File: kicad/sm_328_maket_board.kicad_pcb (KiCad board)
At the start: 2 copper layers, 54.7 x 61.7 mm, 301 parts

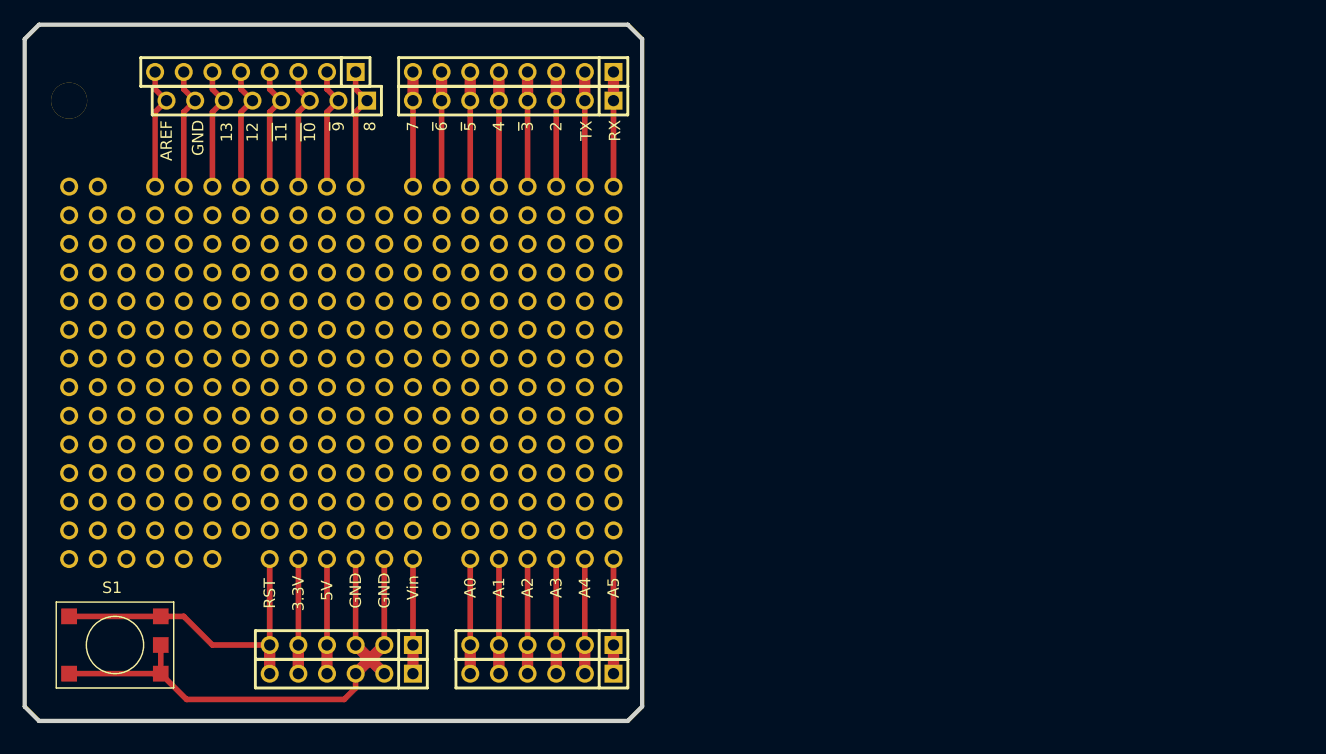
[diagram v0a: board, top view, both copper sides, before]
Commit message: Продолжил разрабатывать макетную плату.
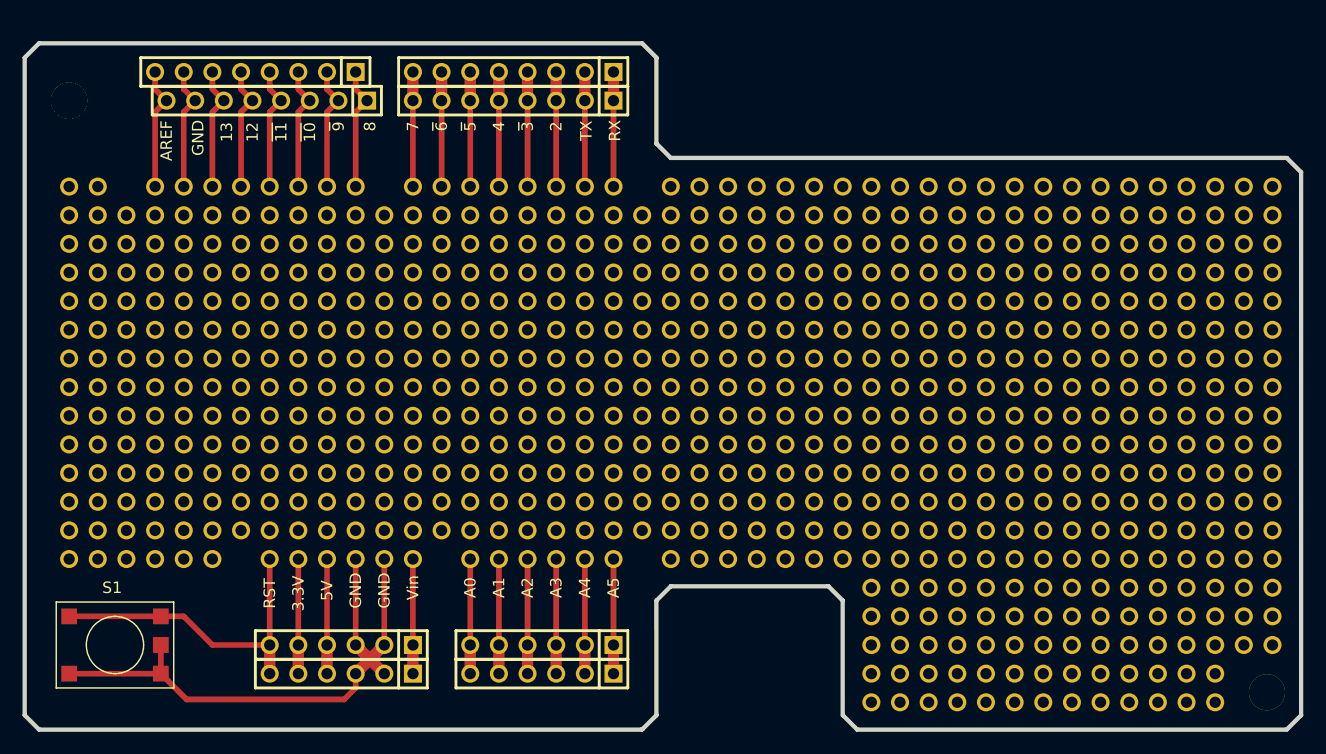
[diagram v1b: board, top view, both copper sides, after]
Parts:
- added G447: P***, 1_pin, F.Cu at (191.0, 139.1)
- added arduino: P***, 1_pin, F.Cu at (175.3, 130.8)
- added arduino: P***, 1_pin, F.Cu at (182.9, 108.0)
- added arduino: P***, 1_pin, F.Cu at (142.2, 123.2)
- added arduino: P***, 1_pin, F.Cu at (193.0, 113.0)
- added arduino: P***, 1_pin, F.Cu at (193.0, 108.0)
- added arduino: P***, 1_pin, F.Cu at (185.4, 97.8)
- added arduino: P***, 1_pin, F.Cu at (154.9, 113.0)
- added arduino: P***, 1_pin, F.Cu at (165.1, 118.1)
- added arduino: P***, 1_pin, F.Cu at (162.6, 113.0)
- added arduino: P***, 1_pin, F.Cu at (180.3, 113.0)
- added arduino: P***, 1_pin, F.Cu at (147.3, 110.5)
- added arduino: P***, 1_pin, F.Cu at (147.3, 108.0)
- added arduino: P***, 1_pin, F.Cu at (167.6, 125.7)
- added arduino: P***, 1_pin, F.Cu at (160.0, 110.5)
- added arduino: P***, 1_pin, F.Cu at (180.3, 118.1)
- added arduino: P***, 1_pin, F.Cu at (149.9, 120.7)
- added arduino: P***, 1_pin, F.Cu at (177.8, 95.2)
- added arduino: P***, 1_pin, F.Cu at (172.7, 120.7)
- added arduino: P***, 1_pin, F.Cu at (188.0, 95.2)
- added arduino: P***, 1_pin, F.Cu at (188.0, 97.8)
- added arduino: P***, 1_pin, F.Cu at (162.6, 100.3)
- added arduino: P***, 1_pin, F.Cu at (144.8, 115.6)
- added arduino: P***, 1_pin, F.Cu at (195.6, 125.7)
- added arduino: P***, 1_pin, F.Cu at (170.2, 130.8)
- added arduino: P***, 1_pin, F.Cu at (147.3, 125.7)
- added arduino: P***, 1_pin, F.Cu at (152.4, 113.0)
- added arduino: P***, 1_pin, F.Cu at (162.6, 135.9)
- added arduino: P***, 1_pin, F.Cu at (170.2, 115.6)
- added arduino: P***, 1_pin, F.Cu at (162.6, 110.5)
- added arduino: P***, 1_pin, F.Cu at (167.6, 113.0)
- added arduino: P***, 1_pin, F.Cu at (165.1, 125.7)
- added arduino: P***, 1_pin, F.Cu at (149.9, 108.0)
- added arduino: P***, 1_pin, F.Cu at (154.9, 108.0)
- added arduino: P***, 1_pin, F.Cu at (170.2, 141.0)
- added arduino: P***, 1_pin, F.Cu at (177.8, 97.8)
- added arduino: P***, 1_pin, F.Cu at (185.4, 130.8)
- added arduino: P***, 1_pin, F.Cu at (157.5, 105.4)
- added arduino: P***, 1_pin, F.Cu at (167.6, 141.0)
- added arduino: P***, 1_pin, F.Cu at (166.6, 109.7)
- added arduino: P***, 1_pin, F.Cu at (172.7, 115.6)
- added arduino: P***, 1_pin, F.Cu at (156.5, 109.7)
- added arduino: P***, 1_pin, F.Cu at (180.3, 133.3)
- added arduino: P***, 1_pin, F.Cu at (195.6, 135.9)
- added arduino: P***, 1_pin, F.Cu at (182.9, 95.2)
- added arduino: P***, 1_pin, F.Cu at (190.5, 108.0)
- added arduino: P***, 1_pin, F.Cu at (182.9, 118.1)
- added arduino: P***, 1_pin, F.Cu at (160.0, 120.7)
- added arduino: P***, 1_pin, F.Cu at (160.0, 133.3)
- added arduino: P***, 1_pin, F.Cu at (182.9, 123.2)
- added arduino: P***, 1_pin, F.Cu at (185.4, 123.2)
- added arduino: P***, 1_pin, F.Cu at (165.1, 105.4)
- added arduino: P***, 1_pin, F.Cu at (160.0, 95.2)
- added arduino: P***, 1_pin, F.Cu at (195.6, 100.3)
- added arduino: P***, 1_pin, F.Cu at (188.0, 110.5)
- added arduino: P***, 1_pin, F.Cu at (154.9, 97.8)
- added arduino: P***, 1_pin, F.Cu at (190.5, 113.0)
- added arduino: P***, 1_pin, F.Cu at (152.4, 100.3)
- added arduino: P***, 1_pin, F.Cu at (152.4, 95.2)
- added arduino: P***, 1_pin, F.Cu at (190.5, 141.0)
- added arduino: P***, 1_pin, F.Cu at (172.7, 123.2)
- added arduino: P***, 1_pin, F.Cu at (177.8, 133.3)
- added arduino: P***, 1_pin, F.Cu at (180.3, 128.3)
- added arduino: P***, 1_pin, F.Cu at (160.0, 138.4)
- added arduino: P***, 1_pin, F.Cu at (190.5, 105.4)
- added arduino: P***, 1_pin, F.Cu at (142.2, 110.5)
- added arduino: P***, 1_pin, F.Cu at (160.0, 108.0)
- added arduino: P***, 1_pin, F.Cu at (190.5, 115.6)
- added arduino: P***, 1_pin, F.Cu at (142.2, 113.0)
- added arduino: P***, 1_pin, F.Cu at (185.4, 120.7)
- added arduino: P***, 1_pin, F.Cu at (152.4, 102.9)
- added arduino: P***, 1_pin, F.Cu at (195.6, 108.0)
- added arduino: P***, 1_pin, F.Cu at (185.4, 95.2)
- added arduino: P***, 1_pin, F.Cu at (195.6, 97.8)
- added arduino: P***, 1_pin, F.Cu at (188.0, 108.0)
- added arduino: P***, 1_pin, F.Cu at (167.6, 135.9)
- added arduino: P***, 1_pin, F.Cu at (139.7, 123.2)
- added arduino: P***, 1_pin, F.Cu at (147.3, 113.0)
- added arduino: P***, 1_pin, F.Cu at (185.4, 118.1)
- added arduino: P***, 1_pin, F.Cu at (165.1, 138.4)
- added arduino: P***, 1_pin, F.Cu at (193.0, 100.3)
- added arduino: P***, 1_pin, F.Cu at (180.3, 105.4)
- added arduino: P***, 1_pin, F.Cu at (185.4, 105.4)
- added arduino: P***, 1_pin, F.Cu at (167.6, 110.5)
- added arduino: P***, 1_pin, F.Cu at (149.9, 128.3)
- added arduino: P***, 1_pin, F.Cu at (193.0, 97.8)
- added arduino: P***, 1_pin, F.Cu at (188.0, 130.8)
- added arduino: P***, 1_pin, F.Cu at (167.6, 133.3)
- added arduino: P***, 1_pin, F.Cu at (167.6, 130.8)
- added arduino: P***, 1_pin, F.Cu at (165.1, 113.0)
- added arduino: P***, 1_pin, F.Cu at (175.3, 138.4)
- added arduino: P***, 1_pin, F.Cu at (175.3, 125.7)
- added arduino: P***, 1_pin, F.Cu at (171.7, 109.7)
- added arduino: P***, 1_pin, F.Cu at (177.8, 141.0)
- added arduino: P***, 1_pin, F.Cu at (147.3, 128.3)
- added arduino: P***, 1_pin, F.Cu at (169.2, 109.7)
- added arduino: P***, 1_pin, F.Cu at (177.8, 105.4)
- added arduino: P***, 1_pin, F.Cu at (160.0, 100.3)
- added arduino: P***, 1_pin, F.Cu at (157.5, 108.0)
- added arduino: P***, 1_pin, F.Cu at (175.3, 123.2)
- added arduino: P***, 1_pin, F.Cu at (185.4, 110.5)
- added arduino: P***, 1_pin, F.Cu at (177.8, 113.0)
- added arduino: P***, 1_pin, F.Cu at (175.3, 95.2)
- added arduino: P***, 1_pin, F.Cu at (142.2, 95.2)
- added arduino: P***, 1_pin, F.Cu at (142.2, 125.7)
- added arduino: P***, 1_pin, F.Cu at (177.8, 115.6)
- added arduino: P***, 1_pin, F.Cu at (188.0, 115.6)
- added arduino: P***, 1_pin, F.Cu at (157.5, 95.2)
- added arduino: P***, 1_pin, F.Cu at (149.9, 113.0)
- added arduino: P***, 1_pin, F.Cu at (185.4, 108.0)
- added arduino: P***, 1_pin, F.Cu at (177.8, 138.4)
- added arduino: P***, 1_pin, F.Cu at (185.4, 125.7)
- added arduino: P***, 1_pin, F.Cu at (157.5, 120.7)
- added arduino: P***, 1_pin, F.Cu at (160.0, 115.6)
- added arduino: P***, 1_pin, F.Cu at (164.1, 109.7)
- added arduino: P***, 1_pin, F.Cu at (184.4, 109.7)
- added arduino: P***, 1_pin, F.Cu at (167.6, 100.3)
- added arduino: P***, 1_pin, F.Cu at (193.0, 125.7)
- added arduino: P***, 1_pin, F.Cu at (165.1, 141.0)
- added arduino: P***, 1_pin, F.Cu at (190.5, 130.8)
- added arduino: P***, 1_pin, F.Cu at (180.3, 108.0)
- added arduino: P***, 1_pin, F.Cu at (175.3, 102.9)
- added arduino: P***, 1_pin, F.Cu at (162.6, 138.4)
- added arduino: P***, 1_pin, F.Cu at (180.3, 120.7)
- added arduino: P***, 1_pin, F.Cu at (152.4, 125.7)
- added arduino: P***, 1_pin, F.Cu at (177.8, 108.0)
- added arduino: P***, 1_pin, F.Cu at (165.1, 123.2)
- added arduino: P***, 1_pin, F.Cu at (182.9, 135.9)
- added arduino: P***, 1_pin, F.Cu at (157.5, 123.2)
- added arduino: P***, 1_pin, F.Cu at (180.3, 141.0)
- added arduino: P***, 1_pin, F.Cu at (182.9, 105.4)
- added arduino: P***, 1_pin, F.Cu at (170.2, 102.9)
- added arduino: P***, 1_pin, F.Cu at (170.2, 128.3)
- added arduino: P***, 1_pin, F.Cu at (185.4, 102.9)
- added arduino: P***, 1_pin, F.Cu at (186.9, 109.7)
- added arduino: P***, 1_pin, F.Cu at (185.4, 113.0)
- added arduino: P***, 1_pin, F.Cu at (182.9, 115.6)
- added arduino: P***, 1_pin, F.Cu at (172.7, 135.9)
- added arduino: P***, 1_pin, F.Cu at (162.6, 130.8)
- added arduino: P***, 1_pin, F.Cu at (89.7, 87.6)
- added arduino: P***, 1_pin, F.Cu at (144.8, 128.3)
- added arduino: P***, 1_pin, F.Cu at (180.3, 110.5)
- added arduino: P***, 1_pin, F.Cu at (149.9, 110.5)
- added arduino: P***, 1_pin, F.Cu at (162.6, 120.7)
- added arduino: P***, 1_pin, F.Cu at (180.3, 123.2)
- added arduino: P***, 1_pin, F.Cu at (144.8, 95.2)
- added arduino: P***, 1_pin, F.Cu at (157.5, 115.6)
- added arduino: P***, 1_pin, F.Cu at (180.3, 138.4)
- added arduino: P***, 1_pin, F.Cu at (193.0, 120.7)
- added arduino: P***, 1_pin, F.Cu at (147.3, 115.6)
- added arduino: P***, 1_pin, F.Cu at (152.4, 118.1)
- added arduino: P***, 1_pin, F.Cu at (144.8, 110.5)
- added arduino: P***, 1_pin, F.Cu at (170.2, 123.2)
- added arduino: P***, 1_pin, F.Cu at (180.3, 95.2)
- added arduino: P***, 1_pin, F.Cu at (188.0, 102.9)
- added arduino: P***, 1_pin, F.Cu at (195.6, 105.4)
- added arduino: P***, 1_pin, F.Cu at (167.6, 118.1)
- added arduino: P***, 1_pin, F.Cu at (165.1, 135.9)
- added arduino: P***, 1_pin, F.Cu at (194.6, 109.7)
- added arduino: P***, 1_pin, F.Cu at (142.2, 102.9)
- added arduino: P***, 1_pin, F.Cu at (190.5, 100.3)
- added arduino: P***, 1_pin, F.Cu at (195.6, 128.3)
- added arduino: P***, 1_pin, F.Cu at (175.3, 108.0)
- added arduino: P***, 1_pin, F.Cu at (165.1, 108.0)
- added arduino: P***, 1_pin, F.Cu at (193.0, 102.9)
- added arduino: P***, 1_pin, F.Cu at (177.8, 125.7)
- added arduino: P***, 1_pin, F.Cu at (162.6, 102.9)
- added arduino: P***, 1_pin, F.Cu at (167.6, 95.2)
- added arduino: P***, 1_pin, F.Cu at (167.6, 115.6)
- added arduino: P***, 1_pin, F.Cu at (139.7, 118.1)
- added arduino: P***, 1_pin, F.Cu at (149.9, 105.4)
- added arduino: P***, 1_pin, F.Cu at (152.4, 128.3)
- added arduino: P***, 1_pin, F.Cu at (180.3, 102.9)
- added arduino: P***, 1_pin, F.Cu at (165.1, 128.3)
- added arduino: P***, 1_pin, F.Cu at (157.5, 128.3)
- added arduino: P***, 1_pin, F.Cu at (144.8, 100.3)
- added arduino: P***, 1_pin, F.Cu at (195.6, 118.1)
- added arduino: P***, 1_pin, F.Cu at (170.2, 97.8)
- added arduino: P***, 1_pin, F.Cu at (149.9, 102.9)
- added arduino: P***, 1_pin, F.Cu at (162.6, 118.1)
- added arduino: P***, 1_pin, F.Cu at (177.8, 135.9)
- added arduino: P***, 1_pin, F.Cu at (177.8, 102.9)
- added arduino: P***, 1_pin, F.Cu at (189.5, 109.7)
- added arduino: P***, 1_pin, F.Cu at (185.4, 115.6)
- added arduino: P***, 1_pin, F.Cu at (182.9, 125.7)
- added arduino: P***, 1_pin, F.Cu at (139.7, 120.7)
- added arduino: P***, 1_pin, F.Cu at (180.3, 115.6)
- added arduino: P***, 1_pin, F.Cu at (177.8, 100.3)
- added arduino: P***, 1_pin, F.Cu at (190.5, 120.7)
- added arduino: P***, 1_pin, F.Cu at (195.6, 115.6)
- added arduino: P***, 1_pin, F.Cu at (170.2, 113.0)
- added arduino: P***, 1_pin, F.Cu at (167.6, 138.4)
- added arduino: P***, 1_pin, F.Cu at (157.5, 118.1)
- added arduino: P***, 1_pin, F.Cu at (152.4, 115.6)
- added arduino: P***, 1_pin, F.Cu at (154.9, 110.5)
- added arduino: P***, 1_pin, F.Cu at (160.0, 141.0)
- added arduino: P***, 1_pin, F.Cu at (182.9, 120.7)
- added arduino: P***, 1_pin, F.Cu at (139.7, 102.9)
- added arduino: P***, 1_pin, F.Cu at (170.2, 138.4)
- added arduino: P***, 1_pin, F.Cu at (185.4, 138.4)
- added arduino: P***, 1_pin, F.Cu at (172.7, 141.0)
- added arduino: P***, 1_pin, F.Cu at (175.3, 113.0)
- added arduino: P***, 1_pin, F.Cu at (190.5, 135.9)
- added arduino: P***, 1_pin, F.Cu at (193.0, 105.4)
- added arduino: P***, 1_pin, F.Cu at (188.0, 141.0)
- added arduino: P***, 1_pin, F.Cu at (160.0, 118.1)
- added arduino: P***, 1_pin, F.Cu at (154.9, 118.1)
- added arduino: P***, 1_pin, F.Cu at (157.5, 100.3)
- added arduino: P***, 1_pin, F.Cu at (144.8, 102.9)
- added arduino: P***, 1_pin, F.Cu at (160.0, 135.9)
- added arduino: P***, 1_pin, F.Cu at (162.6, 97.8)
- added arduino: P***, 1_pin, F.Cu at (157.5, 125.7)
- added arduino: P***, 1_pin, F.Cu at (162.6, 95.2)
- added arduino: P***, 1_pin, F.Cu at (149.9, 100.3)
- added arduino: P***, 1_pin, F.Cu at (167.6, 120.7)
- added arduino: P***, 1_pin, F.Cu at (179.3, 109.7)
- added arduino: P***, 1_pin, F.Cu at (190.5, 102.9)
- added arduino: P***, 1_pin, F.Cu at (139.7, 110.5)
- added arduino: P***, 1_pin, F.Cu at (170.2, 105.4)
- added arduino: P***, 1_pin, F.Cu at (181.9, 109.7)
- added arduino: P***, 1_pin, F.Cu at (188.0, 123.2)
- added arduino: P***, 1_pin, F.Cu at (180.3, 100.3)
- added arduino: P***, 1_pin, F.Cu at (157.5, 97.8)
- added arduino: P***, 1_pin, F.Cu at (182.9, 133.3)
- added arduino: P***, 1_pin, F.Cu at (193.0, 135.9)
- added arduino: P***, 1_pin, F.Cu at (152.4, 97.8)
- added arduino: P***, 1_pin, F.Cu at (175.3, 141.0)
- added arduino: P***, 1_pin, F.Cu at (177.8, 123.2)
- added arduino: P***, 1_pin, F.Cu at (142.2, 100.3)
- added arduino: P***, 1_pin, F.Cu at (167.6, 105.4)
- added arduino: P***, 1_pin, F.Cu at (188.0, 135.9)
- added arduino: P***, 1_pin, F.Cu at (185.4, 100.3)
- added arduino: P***, 1_pin, F.Cu at (188.0, 113.0)
- added arduino: P***, 1_pin, F.Cu at (185.4, 133.3)
- added arduino: P***, 1_pin, F.Cu at (188.0, 133.3)
- added arduino: P***, 1_pin, F.Cu at (162.6, 128.3)
- added arduino: P***, 1_pin, F.Cu at (142.2, 105.4)
- added arduino: P***, 1_pin, F.Cu at (139.7, 115.6)
- added arduino: P***, 1_pin, F.Cu at (185.4, 135.9)
- added arduino: P***, 1_pin, F.Cu at (175.3, 128.3)
- added arduino: P***, 1_pin, F.Cu at (162.6, 133.3)
- added arduino: P***, 1_pin, F.Cu at (138.7, 109.7)
- added arduino: P***, 1_pin, F.Cu at (188.0, 120.7)
- added arduino: P***, 1_pin, F.Cu at (195.6, 130.8)
- added arduino: P***, 1_pin, F.Cu at (182.9, 110.5)
- added arduino: P***, 1_pin, F.Cu at (165.1, 102.9)
- added arduino: P***, 1_pin, F.Cu at (165.1, 120.7)
- added arduino: P***, 1_pin, F.Cu at (149.9, 123.2)
- added arduino: P***, 1_pin, F.Cu at (182.9, 100.3)
- added arduino: P***, 1_pin, F.Cu at (188.0, 128.3)
- added arduino: P***, 1_pin, F.Cu at (188.0, 138.4)
- added arduino: P***, 1_pin, F.Cu at (142.2, 128.3)
- added arduino: P***, 1_pin, F.Cu at (142.2, 115.6)
- added arduino: P***, 1_pin, F.Cu at (162.6, 123.2)
- added arduino: P***, 1_pin, F.Cu at (170.2, 100.3)
- added arduino: P***, 1_pin, F.Cu at (165.1, 100.3)
- added arduino: P***, 1_pin, F.Cu at (170.2, 110.5)
- added arduino: P***, 1_pin, F.Cu at (154.9, 125.7)
- added arduino: P***, 1_pin, F.Cu at (147.3, 120.7)
- added arduino: P***, 1_pin, F.Cu at (177.8, 130.8)
- added arduino: P***, 1_pin, F.Cu at (147.3, 97.8)
- added arduino: P***, 1_pin, F.Cu at (143.8, 109.7)
- added arduino: P***, 1_pin, F.Cu at (139.7, 105.4)
- added arduino: P***, 1_pin, F.Cu at (175.3, 118.1)
- added arduino: P***, 1_pin, F.Cu at (154.9, 100.3)
- added arduino: P***, 1_pin, F.Cu at (180.3, 97.8)
- added arduino: P***, 1_pin, F.Cu at (147.3, 100.3)
- added arduino: P***, 1_pin, F.Cu at (172.7, 105.4)
- added arduino: P***, 1_pin, F.Cu at (177.8, 118.1)
- added arduino: P***, 1_pin, F.Cu at (162.6, 125.7)
- added arduino: P***, 1_pin, F.Cu at (160.0, 102.9)
- added arduino: P***, 1_pin, F.Cu at (144.8, 125.7)
- added arduino: P***, 1_pin, F.Cu at (188.0, 100.3)
- added arduino: P***, 1_pin, F.Cu at (193.0, 123.2)
- added arduino: P***, 1_pin, F.Cu at (144.8, 97.8)
- added arduino: P***, 1_pin, F.Cu at (149.9, 97.8)
- added arduino: P***, 1_pin, F.Cu at (195.6, 123.2)
- added arduino: P***, 1_pin, F.Cu at (190.5, 110.5)
- added arduino: P***, 1_pin, F.Cu at (172.7, 95.2)
- added arduino: P***, 1_pin, F.Cu at (190.5, 133.3)
- added arduino: P***, 1_pin, F.Cu at (162.6, 108.0)
- added arduino: P***, 1_pin, F.Cu at (172.7, 108.0)
- added arduino: P***, 1_pin, F.Cu at (170.2, 135.9)
- added arduino: P***, 1_pin, F.Cu at (160.0, 105.4)
- added arduino: P***, 1_pin, F.Cu at (190.5, 123.2)
- added arduino: P***, 1_pin, F.Cu at (170.2, 118.1)
- added arduino: P***, 1_pin, F.Cu at (165.1, 115.6)
- added arduino: P***, 1_pin, F.Cu at (195.6, 113.0)
- added arduino: P***, 1_pin, F.Cu at (175.3, 100.3)
- added arduino: P***, 1_pin, F.Cu at (149.9, 95.2)
- added arduino: P***, 1_pin, F.Cu at (190.5, 95.2)
- added arduino: P***, 1_pin, F.Cu at (154.9, 123.2)
- added arduino: P***, 1_pin, F.Cu at (160.0, 113.0)
- added arduino: P***, 1_pin, F.Cu at (172.7, 128.3)
- added arduino: P***, 1_pin, F.Cu at (185.4, 141.0)
- added arduino: P***, 1_pin, F.Cu at (175.3, 110.5)
- added arduino: P***, 1_pin, F.Cu at (154.9, 102.9)
- added arduino: P***, 1_pin, F.Cu at (167.6, 102.9)
- added arduino: P***, 1_pin, F.Cu at (175.3, 115.6)
- added arduino: P***, 1_pin, F.Cu at (182.9, 97.8)
- added arduino: P***, 1_pin, F.Cu at (139.7, 108.0)
- added arduino: P***, 1_pin, F.Cu at (147.3, 118.1)
- added arduino: P***, 1_pin, F.Cu at (167.6, 97.8)
- added arduino: P***, 1_pin, F.Cu at (172.7, 97.8)
- added arduino: P***, 1_pin, F.Cu at (146.3, 109.7)
- added arduino: P***, 1_pin, F.Cu at (192.0, 109.7)
- added arduino: P***, 1_pin, F.Cu at (144.8, 118.1)
- added arduino: P***, 1_pin, F.Cu at (190.5, 138.4)
- added arduino: P***, 1_pin, F.Cu at (185.4, 128.3)
- added arduino: P***, 1_pin, F.Cu at (182.9, 138.4)
- added arduino: P***, 1_pin, F.Cu at (195.6, 95.2)
- added arduino: P***, 1_pin, F.Cu at (188.0, 125.7)
- added arduino: P***, 1_pin, F.Cu at (195.6, 120.7)
- added arduino: P***, 1_pin, F.Cu at (165.1, 97.8)
- added arduino: P***, 1_pin, F.Cu at (193.0, 95.2)
- added arduino: P***, 1_pin, F.Cu at (172.7, 118.1)
- added arduino: P***, 1_pin, F.Cu at (152.4, 110.5)
- added arduino: P***, 1_pin, F.Cu at (193.0, 128.3)
- added arduino: P***, 1_pin, F.Cu at (154.9, 105.4)
- added arduino: P***, 1_pin, F.Cu at (160.0, 130.8)
- added arduino: P***, 1_pin, F.Cu at (144.8, 120.7)
- added arduino: P***, 1_pin, F.Cu at (193.0, 110.5)
- added arduino: P***, 1_pin, F.Cu at (177.8, 110.5)
- added arduino: P***, 1_pin, F.Cu at (162.6, 141.0)
- added arduino: P***, 1_pin, F.Cu at (151.4, 109.7)
- added arduino: P***, 1_pin, F.Cu at (172.7, 110.5)
- added arduino: P***, 1_pin, F.Cu at (157.5, 110.5)
- added arduino: P***, 1_pin, F.Cu at (182.9, 128.3)
- added arduino: P***, 1_pin, F.Cu at (147.3, 95.2)
- added arduino: P***, 1_pin, F.Cu at (175.3, 97.8)
- added arduino: P***, 1_pin, F.Cu at (141.2, 109.7)
- added arduino: P***, 1_pin, F.Cu at (165.1, 130.8)
- added arduino: P***, 1_pin, F.Cu at (157.5, 102.9)
- added arduino: P***, 1_pin, F.Cu at (175.3, 120.7)
- added arduino: P***, 1_pin, F.Cu at (160.0, 128.3)
- added arduino: P***, 1_pin, F.Cu at (144.8, 105.4)
- added arduino: P***, 1_pin, F.Cu at (139.7, 113.0)
- added arduino: P***, 1_pin, F.Cu at (172.7, 138.4)
- added arduino: P***, 1_pin, F.Cu at (172.7, 133.3)
- added arduino: P***, 1_pin, F.Cu at (170.2, 120.7)
- added arduino: P***, 1_pin, F.Cu at (180.3, 125.7)
- added arduino: P***, 1_pin, F.Cu at (144.8, 123.2)
- added arduino: P***, 1_pin, F.Cu at (149.9, 115.6)
- added arduino: P***, 1_pin, F.Cu at (167.6, 108.0)
- added arduino: P***, 1_pin, F.Cu at (188.0, 118.1)
- added arduino: P***, 1_pin, F.Cu at (175.3, 133.3)
- added arduino: P***, 1_pin, F.Cu at (152.4, 123.2)
- added arduino: P***, 1_pin, F.Cu at (182.9, 113.0)
- added arduino: P***, 1_pin, F.Cu at (167.6, 128.3)
- added arduino: P***, 1_pin, F.Cu at (190.5, 125.7)
- added arduino: P***, 1_pin, F.Cu at (144.8, 108.0)
- added arduino: P***, 1_pin, F.Cu at (182.9, 130.8)
- added arduino: P***, 1_pin, F.Cu at (148.8, 109.7)
- added arduino: P***, 1_pin, F.Cu at (160.0, 125.7)
- added arduino: P***, 1_pin, F.Cu at (139.7, 97.8)
- added arduino: P***, 1_pin, F.Cu at (153.9, 109.7)
- added arduino: P***, 1_pin, F.Cu at (190.5, 97.8)
- added arduino: P***, 1_pin, F.Cu at (149.9, 118.1)
- added arduino: P***, 1_pin, F.Cu at (142.2, 120.7)
- added arduino: P***, 1_pin, F.Cu at (162.6, 105.4)
- added arduino: P***, 1_pin, F.Cu at (152.4, 108.0)
- added arduino: P***, 1_pin, F.Cu at (165.1, 110.5)
- added arduino: P***, 1_pin, F.Cu at (160.0, 97.8)
- added arduino: P***, 1_pin, F.Cu at (182.9, 102.9)
- added arduino: P***, 1_pin, F.Cu at (180.3, 135.9)
- added arduino: P***, 1_pin, F.Cu at (147.3, 102.9)
- added arduino: P***, 1_pin, F.Cu at (157.5, 113.0)
- added arduino: P***, 1_pin, F.Cu at (162.6, 115.6)
- added arduino: P***, 1_pin, F.Cu at (142.2, 108.0)
- added arduino: P***, 1_pin, F.Cu at (152.4, 105.4)
- added arduino: P***, 1_pin, F.Cu at (193.0, 118.1)
- added arduino: P***, 1_pin, F.Cu at (149.9, 125.7)
- added arduino: P***, 1_pin, F.Cu at (142.2, 97.8)
- added arduino: P***, 1_pin, F.Cu at (172.7, 102.9)
- added arduino: P***, 1_pin, F.Cu at (182.9, 141.0)
- added arduino: P***, 1_pin, F.Cu at (172.7, 130.8)
- added arduino: P***, 1_pin, F.Cu at (172.7, 125.7)
- added arduino: P***, 1_pin, F.Cu at (188.0, 105.4)
- added arduino: P***, 1_pin, F.Cu at (193.0, 133.3)
- added arduino: P***, 1_pin, F.Cu at (170.2, 125.7)
- added arduino: P***, 1_pin, F.Cu at (175.3, 105.4)
- added arduino: P***, 1_pin, F.Cu at (142.2, 118.1)
- added arduino: P***, 1_pin, F.Cu at (190.5, 118.1)
- added arduino: P***, 1_pin, F.Cu at (170.2, 133.3)
- added arduino: P***, 1_pin, F.Cu at (139.7, 125.7)
- added arduino: P***, 1_pin, F.Cu at (193.0, 130.8)
- added arduino: P***, 1_pin, F.Cu at (170.2, 108.0)
- added arduino: P***, 1_pin, F.Cu at (154.9, 120.7)
- added arduino: P***, 1_pin, F.Cu at (161.5, 109.7)
- added arduino: P***, 1_pin, F.Cu at (147.3, 123.2)
- added arduino: P***, 1_pin, F.Cu at (154.9, 128.3)
- added arduino: P***, 1_pin, F.Cu at (170.2, 95.2)
- added arduino: P***, 1_pin, F.Cu at (172.7, 113.0)
- added arduino: P***, 1_pin, F.Cu at (193.0, 115.6)
- added arduino: P***, 1_pin, F.Cu at (177.8, 120.7)
- added arduino: P***, 1_pin, F.Cu at (147.3, 105.4)
- added arduino: P***, 1_pin, F.Cu at (165.1, 133.3)
- added arduino: P***, 1_pin, F.Cu at (195.6, 133.3)
- added arduino: P***, 1_pin, F.Cu at (167.6, 123.2)
- added arduino: P***, 1_pin, F.Cu at (190.5, 128.3)
- added arduino: P***, 1_pin, F.Cu at (152.4, 120.7)
- added arduino: P***, 1_pin, F.Cu at (195.6, 110.5)
- added arduino: P***, 1_pin, F.Cu at (154.9, 115.6)
- added arduino: P***, 1_pin, F.Cu at (195.6, 102.9)
- added arduino: P***, 1_pin, F.Cu at (139.7, 100.3)
- added arduino: P***, 1_pin, F.Cu at (176.8, 109.7)
- added arduino: P***, 1_pin, F.Cu at (160.0, 123.2)
- added arduino: P***, 1_pin, F.Cu at (159.0, 109.7)
- added arduino: P***, 1_pin, F.Cu at (177.8, 128.3)
- added arduino: P***, 1_pin, F.Cu at (172.7, 100.3)
- added arduino: P***, 1_pin, F.Cu at (144.8, 113.0)
- added arduino: P***, 1_pin, F.Cu at (174.2, 109.7)
- added arduino: P***, 1_pin, F.Cu at (154.9, 95.2)
- added arduino: P***, 1_pin, F.Cu at (180.3, 130.8)
- added arduino: P***, 1_pin, F.Cu at (175.3, 135.9)
- added arduino: P***, 1_pin, F.Cu at (165.1, 95.2)
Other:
- board size 54.7 x 61.7 mm -> 113.2 x 60.8 mm
